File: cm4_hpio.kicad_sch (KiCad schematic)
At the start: 10 parts, among them CN10 M2 x 2.5mm, CN9 TE 1-2199230-6

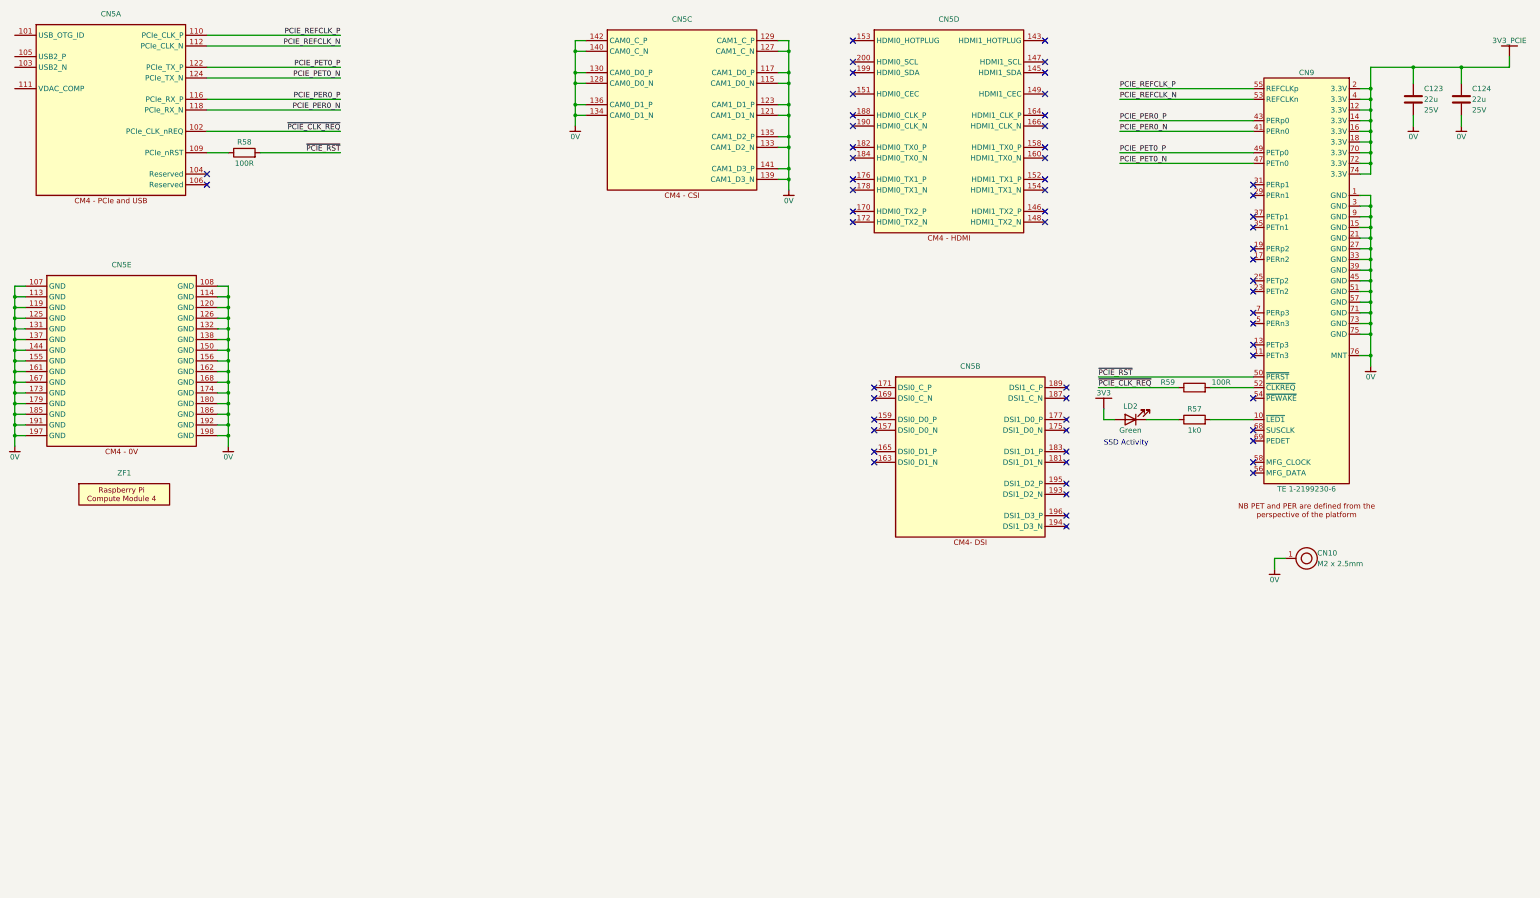
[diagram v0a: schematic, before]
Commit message: started on power
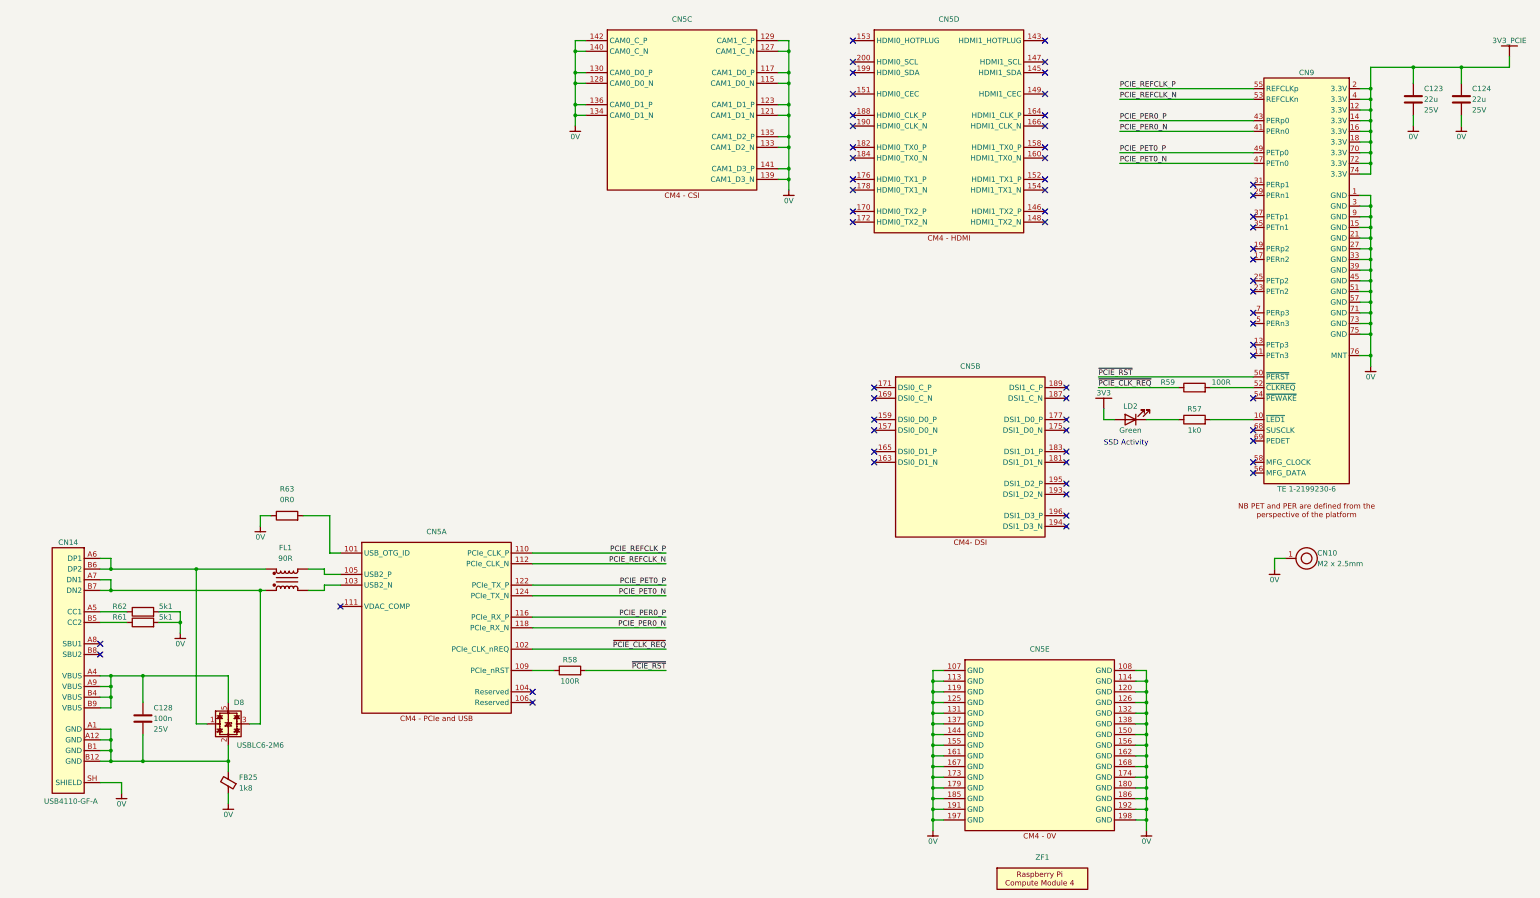
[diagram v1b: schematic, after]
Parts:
- added C128: 100n, Capacitor_SMD:C_0402_1005Metric, symbol Auto_Library_WUT:Yageo CC0402KRX7R8BB104
- added CN14: USB4110-GF-A, Connector_WUT:USB-C_GCT_USB4110-GF-A, symbol Connector_WUT:GCT_USB4110-GF-A
- added D8: USBLC6-2M6, Diode_WUT:TVS_ST_USBLC6-2M6, symbol Diode_WUT:USBLC6-2M6
- added FB25: 1k8, Inductor_SMD:L_0402_1005Metric, symbol Auto_Library_WUT:Murata BLM15BD182SN1D
- added FL1: 90R, Inductor_WUT:L_CommonMode_Wurth_WE-CNSW_0805, symbol Auto_Library_WUT:Wurth Elektronik 744231091
- added R61, R62: 5k1, Resistor_SMD:R_0402_1005Metric, symbol Auto_Library_WUT:KOA Speer RK73H1ETTP5101F
- added R63: 0R0, Resistor_SMD:R_0402_1005Metric, symbol Auto_Library_WUT:KOA Speer RK73Z1ETTP
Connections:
- net 0V: now also CN14.SH (SHIELD), FB25.1, R61.2, R62.2, R63.1
- net at CN5.101 (USB_OTG_ID): now also R63.2
- net at CN5.103 (USB2_N): now also FL1.4
- net at CN5.105 (USB2_P): now also FL1.2
- new net: CN14.A6 (DP1), CN14.B6 (DP2), D8.1, D8.6, FL1.1
- new net: C128.2, CN14.A1 (GND), CN14.A12 (GND), CN14.B1 (GND), CN14.B12 (GND), D8.2, FB25.2
- new net: CN14.A7 (DN1), CN14.B7 (DN2), D8.3, D8.4, FL1.3
- new net: C128.1, CN14.A4 (VBUS), CN14.A9 (VBUS), CN14.B4 (VBUS), CN14.B9 (VBUS), D8.5
- new net: CN14.A5 (CC1), R62.1
- new net: CN14.B5 (CC2), R61.1
- no-connect marks 59 -> 62
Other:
- moved on the sheet: CN5A, CN5E, R58, ZF1

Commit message: Schematic mostly done
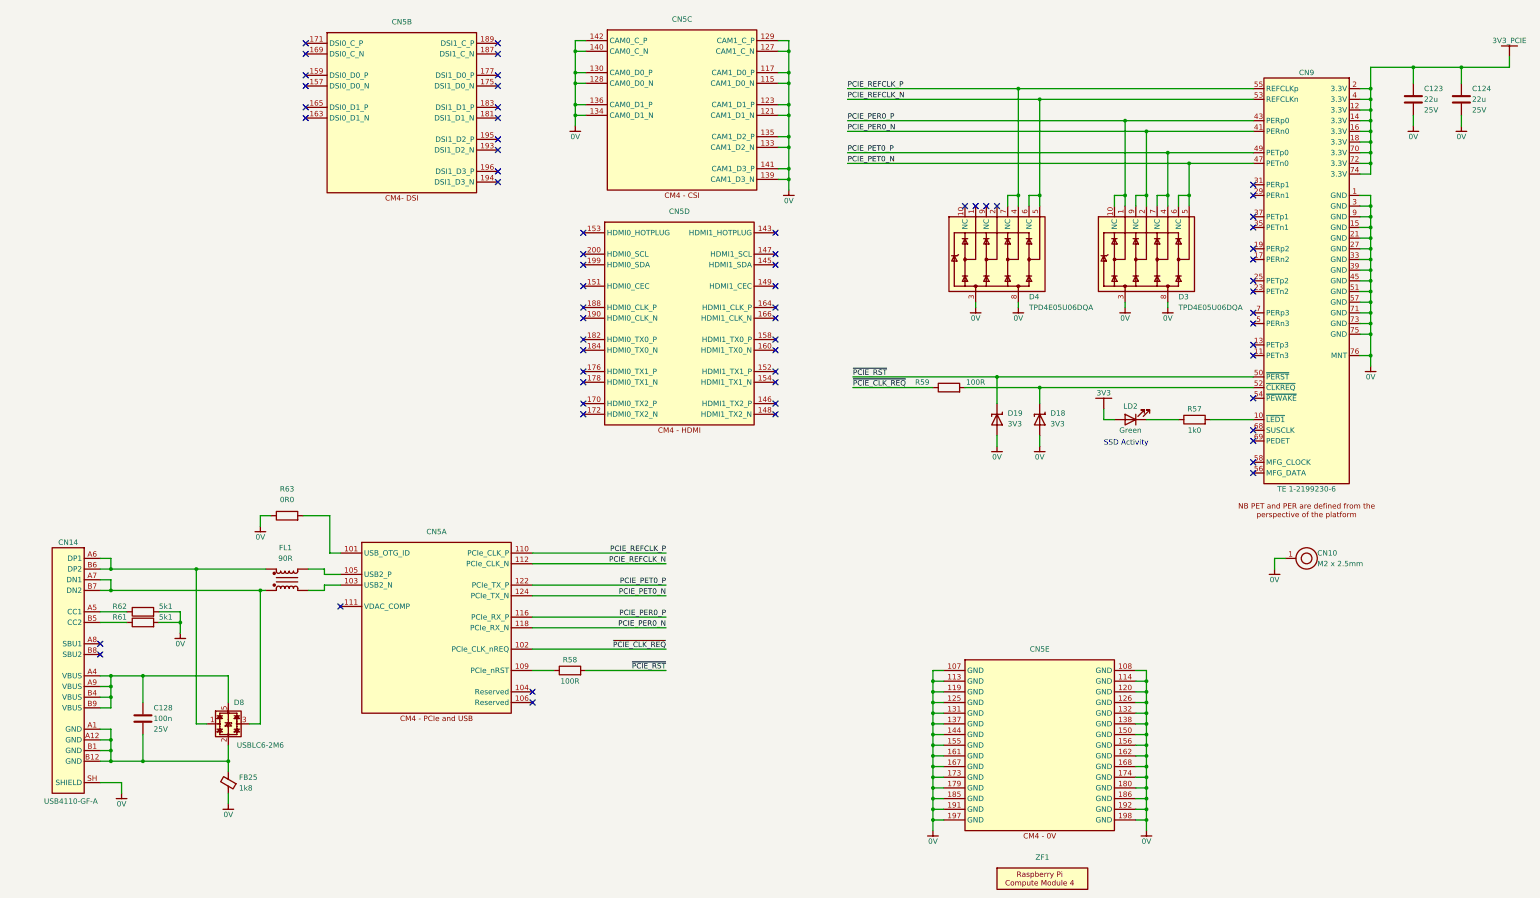
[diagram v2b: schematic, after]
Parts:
- added D18, D19: 3V3, Diode_SMD:D_SOD-523, symbol Auto_Library_WUT:nexperia PESD3V3U1UB,115
- added D3, D4: TPD4E05U06DQA, Diode_WUT:TPD4E05U06DQA, symbol Diode_WUT:TI_TPD4E05U06
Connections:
- net 0V: now also D18.2 (A), D19.2 (A), D3.3, D3.8, D4.3, D4.8
- net PCIE_PER0_N: now also D3.2, D3.9 (NC)
- net PCIE_PER0_P: now also D3.1, D3.10 (NC)
- net PCIE_PET0_N: now also D3.5, D3.6 (NC)
- net PCIE_PET0_P: now also D3.4, D3.7 (NC)
- net PCIE_REFCLK_N: now also D4.5, D4.6 (NC)
- net PCIE_REFCLK_P: now also D4.4, D4.7 (NC)
- net ~{PCIE_RST}: now also D19.1 (K)
- net at CN9.52 (~{CLKREQ}), R59.2: now also D18.1 (K)
- no-connect marks 62 -> 66
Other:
- moved on the sheet: CN5B, CN5D, R59
